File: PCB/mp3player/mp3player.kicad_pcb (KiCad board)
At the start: 2 copper layers, 60 x 85.5 mm, 70 parts, among them J1 AudioJack3, J2 Battery, J3 USB_C, J4 Micro_SD_Card, J5 TFT SPI, SW1 Play, SW10 Power_sw, SW11 Next, SW12 Prev, SW2 Trk Prev, SW3 Trk Next, SW4 Mode Prev, SW5 Mode Next, SW6 Eq, SW7 Power, SW8 RESET, SW9 BOOT, U1 ESP32-S3-WROOM-1, U2 ES8388, U3 AP2112K-3.3, U4 MCP73831-2-OT, U5 USBLC6-2SC6

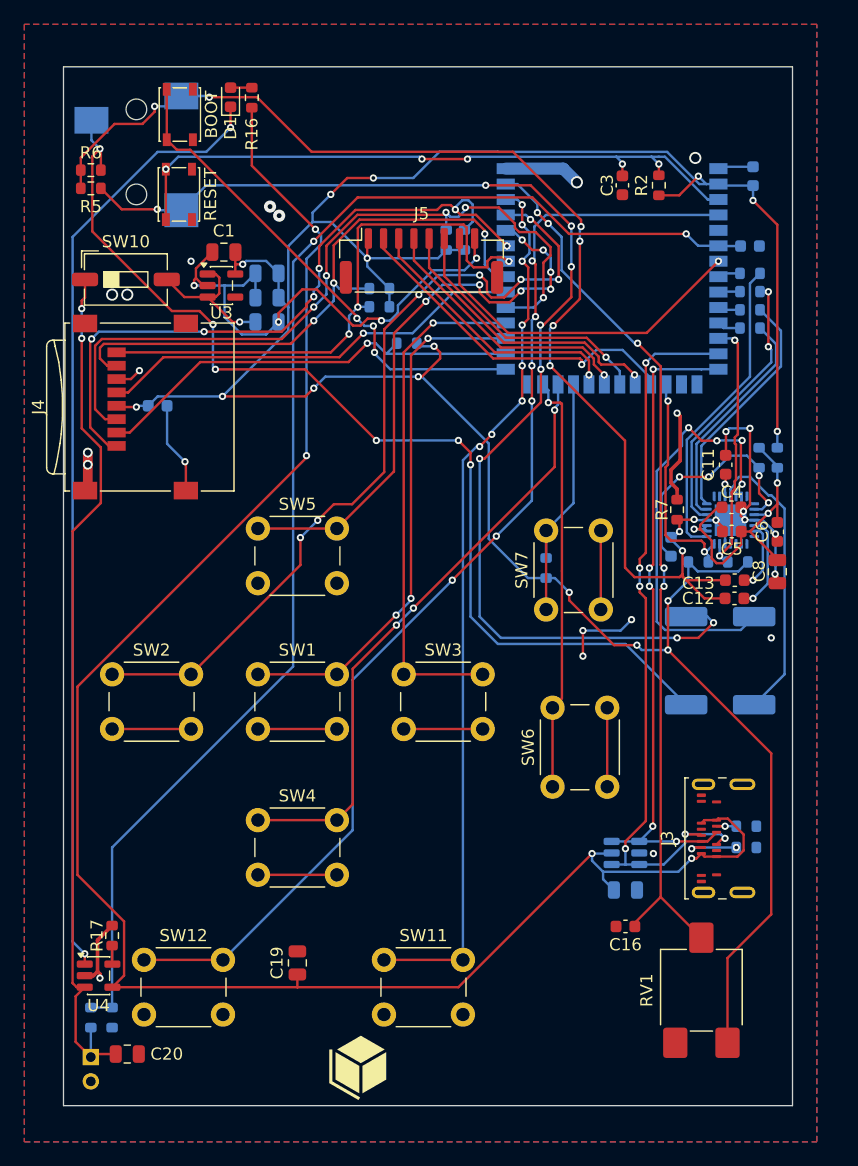
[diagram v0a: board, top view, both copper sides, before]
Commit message: board design
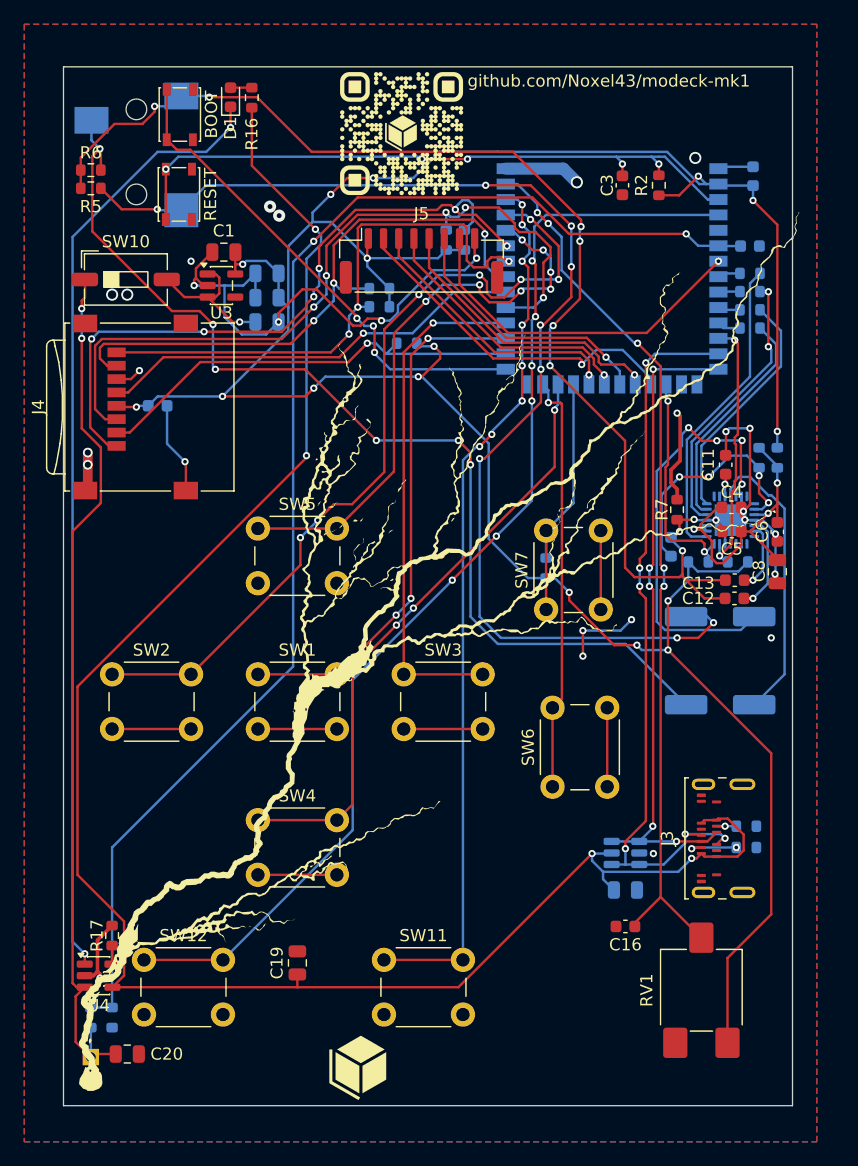
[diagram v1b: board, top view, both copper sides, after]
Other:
- board text added: "github.com/Noxel43/modeck-mk1"
